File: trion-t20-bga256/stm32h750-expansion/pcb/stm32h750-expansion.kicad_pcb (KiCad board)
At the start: 4 copper layers, 48 x 45.5 mm, 77 parts, among them J1 CONN_02x18, J2 CORTEX_DEBUG_ETM, J3 U.FL, J4 U.FL, J5 U.FL, J6 CONN_01X03, J7 CONN_01X03, J8 PMOD_HOST, M1 MECHANICAL, U1 STM32H750XBH6, U2 AT24MAC402, U3 ECS-1612MV-250-CN, U4 W25Q80BV

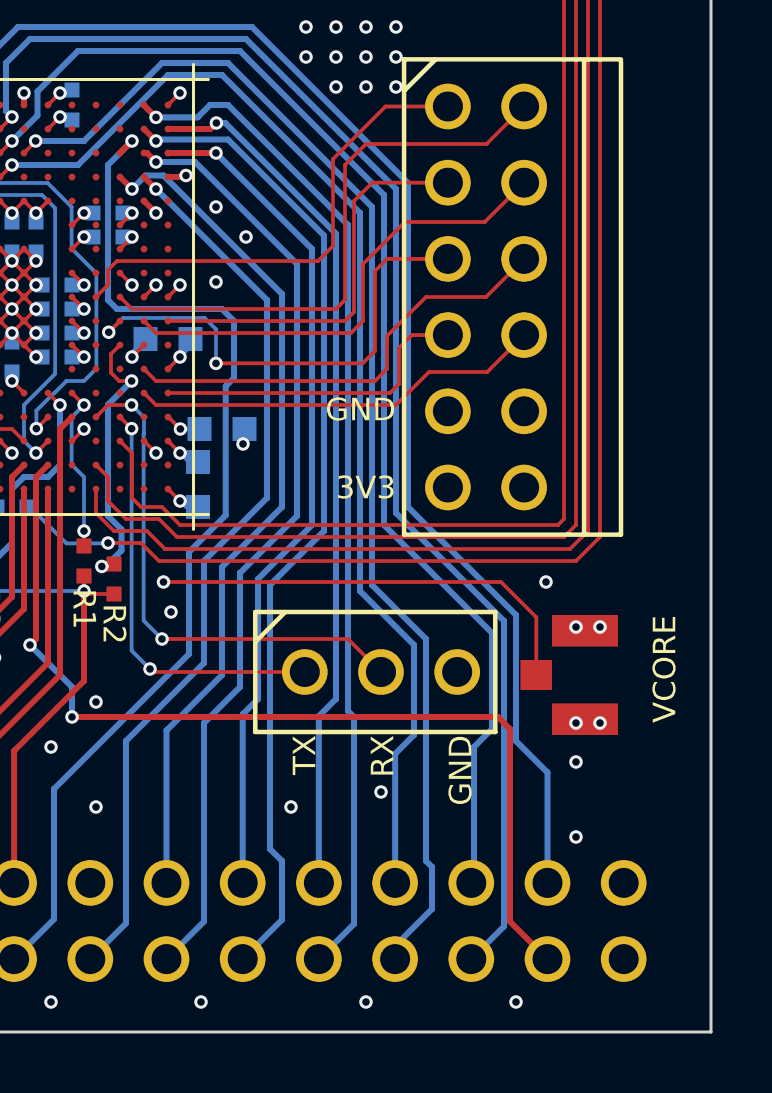
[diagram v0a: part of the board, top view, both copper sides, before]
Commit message: Updated final version of stm32h750-expansion with routing tweaks and export config
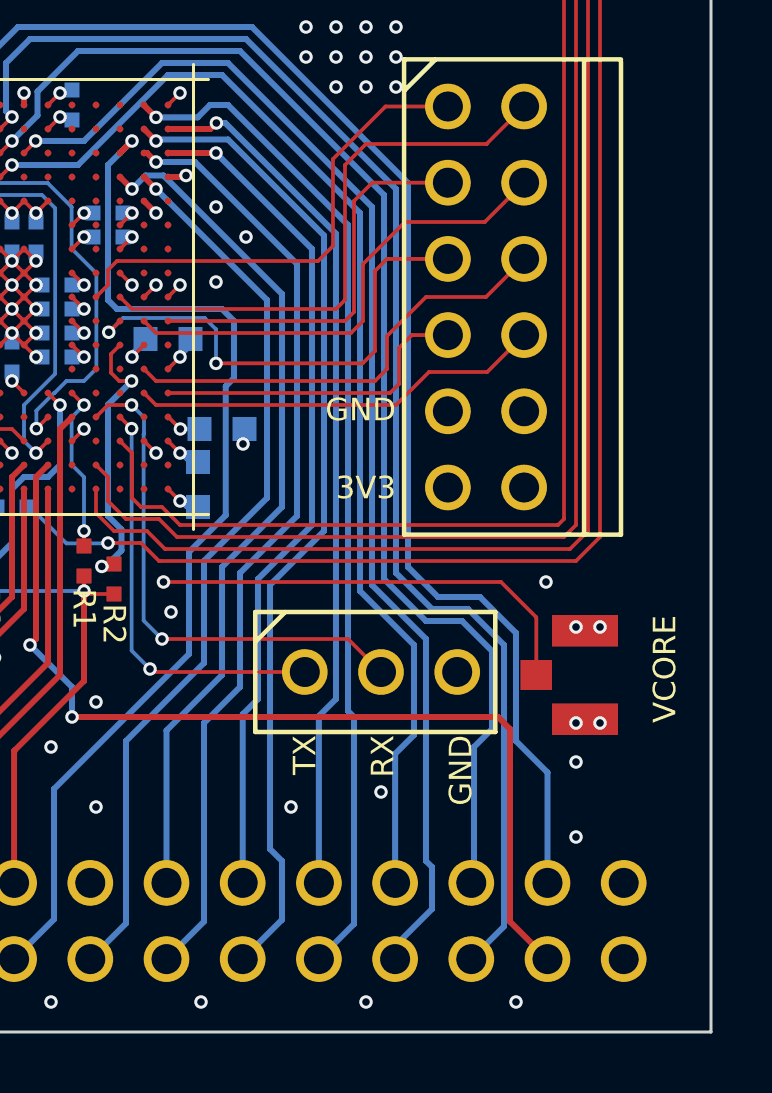
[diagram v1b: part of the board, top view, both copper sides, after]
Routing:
- net /FMC_AD11: track 44.4 -> 45.2 mm
- net /FMC_AD9: track 41.2 -> 41.9 mm
- net /FMC_AD10: track 45.5 -> 46.2 mm
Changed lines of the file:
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@@
 			(outputformat 1)
 			(mirror no)
-			(drillshape 1)
+			(drillshape 0)
 			(scaleselection 1)
-			(outputdirectory "")
+			(outputdirectory "output/")
 		)
 	)
@@
 	)
 	(segment
-		(start 67.6 44.6)
-		(end 67.6 55.6)
+		(start 67.6 57.4)
+		(end 69 58.8)
 		(width 0.2)
 		(layer "B.Cu")
@@
 	)
 	(segment
-		(start 57.4 39.8)
-		(end 62.8 39.8)
+		(start 55.2 42.8)
+		(end 56.05 41.95)
 		(width 0.2)
 		(layer "B.Cu")
@@
 	)
 	(segment
-		(start 56.05 41.95)
-		(end 56.05 41.15)
+		(start 71.2 62.4)
+		(end 70.6 63)
 		(width 0.2)
 		(layer "B.Cu")
@@
 	)
 	(segment
-		(start 67.6 55.6)
-		(end 71.2 59.2)
+		(start 62.8 39.8)
+		(end 67.6 44.6)
 		(width 0.2)
 		(layer "B.Cu")
@@
 	)
 	(segment
-		(start 62.8 39.8)
-		(end 67.6 44.6)
+		(start 69 58.8)
+		(end 70.2 58.8)
 		(width 0.2)
 		(layer "B.Cu")
@@
 	)
 	(segment
-		(start 71.2 59.2)
-		(end 71.2 62.4)
+		(start 67.6 44.6)
+		(end 67.6 57.4)
 		(width 0.2)
 		(layer "B.Cu")
@@
 	)
 	(segment
-		(start 56.05 41.15)
-		(end 57.4 39.8)
+		(start 70.2 58.8)
+		(end 71.2 59.8)
 		(width 0.2)
 		(layer "B.Cu")
@@
 	)
 	(segment
-		(start 55.2 42.8)
-		(end 56.05 41.95)
+		(start 56.05 41.95)
+		(end 56.05 41.15)
 		(width 0.2)
 		(layer "B.Cu")
@@
 	)
 	(segment
-		(start 71.2 62.4)
-		(end 70.6 63)
+		(start 71.2 59.8)
+		(end 71.2 62.4)
+		(width 0.2)
+		(layer "B.Cu")
+		(net 26)
+	)
+	(segment
+		(start 56.05 41.15)
+		(end 57.4 39.8)
+		(width 0.2)
+		(layer "B.Cu")
+		(net 26)
+	)
+	(segment
+		(start 57.4 39.8)
+		(end 62.8 39.8)
 		(width 0.2)
 		(layer "B.Cu")
@@
 	)
 	(segment
-		(start 68.4 44.2)
-		(end 63.2 39)
+		(start 54.4 40)
+		(end 54.4 42)
 		(width 0.2)
 		(layer "B.Cu")
@@
 	)
 	(segment
-		(start 68.4 55)
+		(start 55.4 39)
+		(end 54.4 40)
+		(width 0.2)
+		(layer "B.Cu")
+		(net 31)
+	)
+	(segment
+		(start 68.4 57)
 		(end 68.4 44.2)
 		(width 0.2)
@@
 	)
 	(segment
-		(start 72 58.6)
-		(end 68.4 55)
+		(start 69.4 58)
+		(end 68.4 57)
 		(width 0.2)
 		(layer "B.Cu")
@@
 	)
 	(segment
-		(start 54.4 40)
-		(end 54.4 42)
+		(start 73.05 67.53)
+		(end 73.05 63.85)
 		(width 0.2)
 		(layer "B.Cu")
@@
 	)
 	(segment
-		(start 55.4 39)
-		(end 54.4 40)
+		(start 72 62.8)
+		(end 72 59.2)
 		(width 0.2)
 		(layer "B.Cu")
@@
 	)
 	(segment
-		(start 73.05 67.53)
-		(end 73.05 63.85)
+		(start 70.8 58)
+		(end 69.4 58)
 		(width 0.2)
 		(layer "B.Cu")
@@
 	)
 	(segment
-		(start 63.2 39)
-		(end 55.4 39)
+		(start 72 59.2)
+		(end 70.8 58)
 		(width 0.2)
 		(layer "B.Cu")
@@
 	)
 	(segment
-		(start 72 62.8)
-		(end 72 58.6)
+		(start 68.4 44.2)
+		(end 63.2 39)
+		(width 0.2)
+		(layer "B.Cu")
+		(net 31)
+	)
+	(segment
+		(start 63.2 39)
+		(end 55.4 39)
 		(width 0.2)
 		(layer "B.Cu")
@@
 	)
 	(segment
-		(start 55 41.8)
-		(end 55 40.2)
+		(start 55.2 42)
+		(end 55 41.8)
 		(width 0.2)
 		(layer "B.Cu")
@@
 	)
 	(segment
-		(start 68 55.2)
-		(end 71.6 58.8)
+		(start 55 40.2)
+		(end 55.8 39.4)
 		(width 0.2)
 		(layer "B.Cu")
@@
 	)
 	(segment
-		(start 63 39.4)
-		(end 68 44.4)
+		(start 71.6 68.980001)
+		(end 70.51 70.070001)
 		(width 0.2)
 		(layer "B.Cu")
@@
 	)
 	(segment
-		(start 55 40.2)
-		(end 55.8 39.4)
+		(start 68 57.2)
+		(end 69.2 58.4)
 		(width 0.2)
 		(layer "B.Cu")
@@
 	)
 	(segment
-		(start 71.6 68.980001)
-		(end 70.51 70.070001)
+		(start 68 44.4)
+		(end 68 57.2)
 		(width 0.2)
 		(layer "B.Cu")
@@
 	)
 	(segment
-		(start 55.8 39.4)
-		(end 63 39.4)
+		(start 69.2 58.4)
+		(end 70.4 58.4)
 		(width 0.2)
 		(layer "B.Cu")
@@
 	)
 	(segment
-		(start 71.6 58.8)
-		(end 71.6 68.980001)
+		(start 55 41.8)
+		(end 55 40.2)
 		(width 0.2)
 		(layer "B.Cu")
@@
 	)
 	(segment
-		(start 68 44.4)
-		(end 68 55.2)
+		(start 63 39.4)
+		(end 68 44.4)
 		(width 0.2)
 		(layer "B.Cu")
@@
 	)
 	(segment
-		(start 55.2 42)
-		(end 55 41.8)
+		(start 55.8 39.4)
+		(end 63 39.4)
+		(width 0.2)
+		(layer "B.Cu")
+		(net 37)
+	)
+	(segment
+		(start 70.4 58.4)
+		(end 71.6 59.6)
+		(width 0.2)
+		(layer "B.Cu")
+		(net 37)
+	)
+	(segment
+		(start 71.6 59.6)
+		(end 71.6 68.980001)
 		(width 0.2)
 		(layer "B.Cu")
